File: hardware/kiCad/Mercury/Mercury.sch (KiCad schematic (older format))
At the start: 55 parts

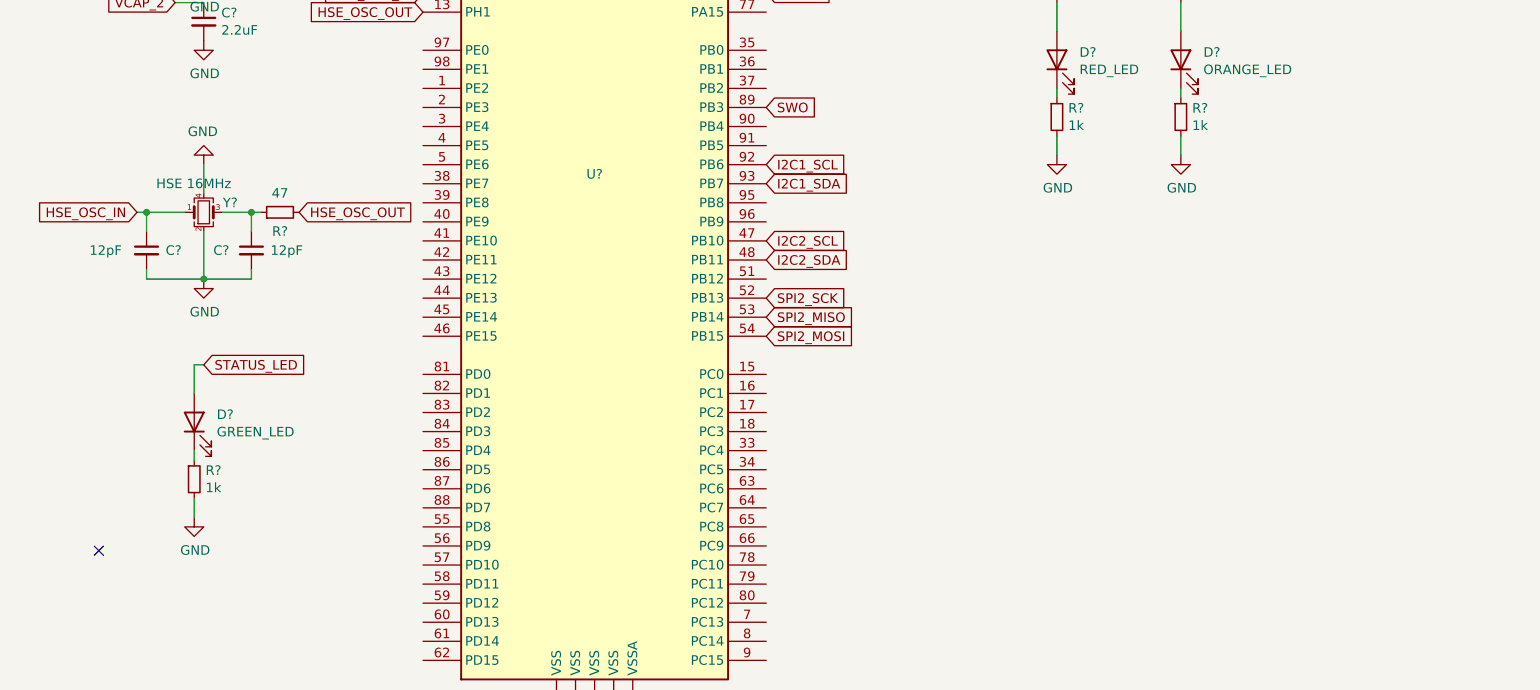
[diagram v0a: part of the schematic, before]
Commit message: Peripherals Added
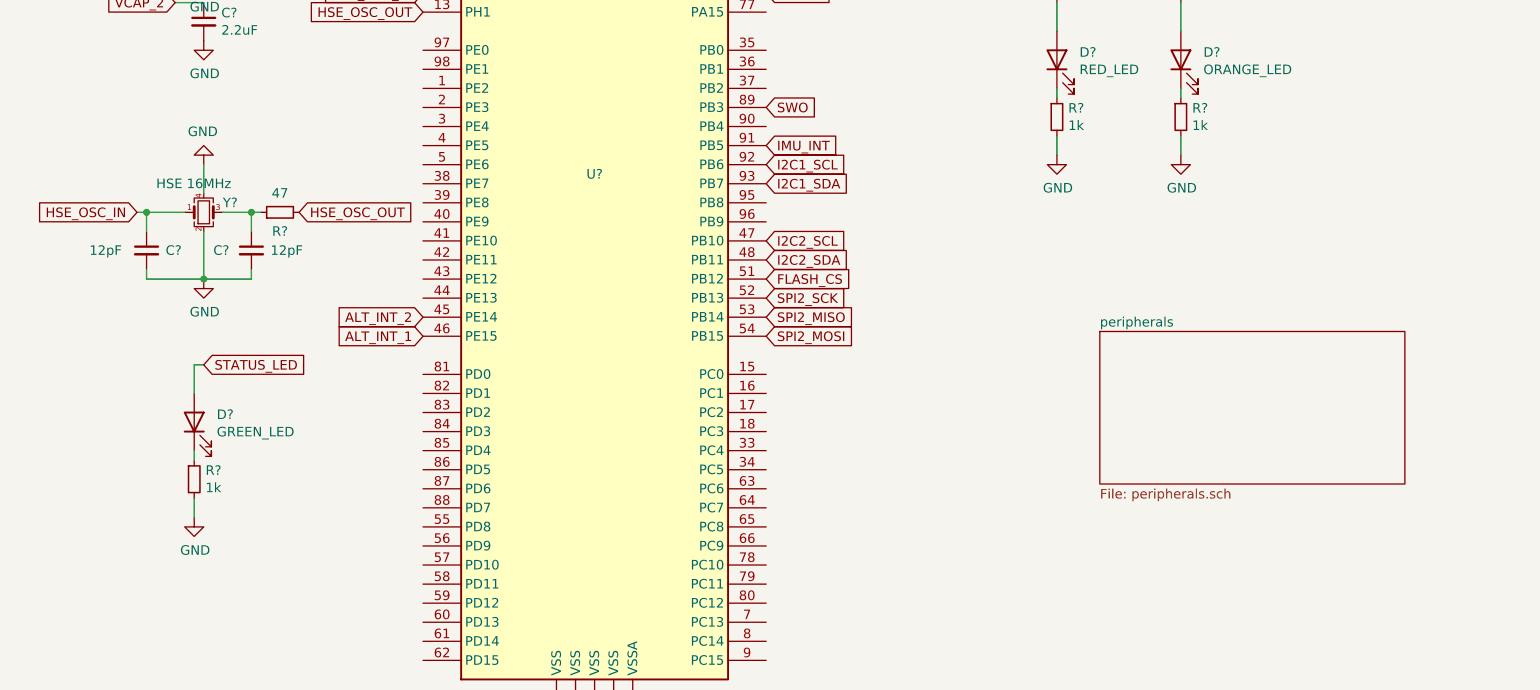
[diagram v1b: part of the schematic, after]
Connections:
- net ALT_INT_2: now reaches U?.45 (PE14)
- net ALT_INT_1: now reaches U?.46 (PE15)
- net FLASH_CS: now reaches U?.51 (PB12)
- net IMU_INT: now reaches U?.91 (PB5)
- no-connect marks 6 -> 5
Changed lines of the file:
@@
 $Descr USLetter 11000 8500
 encoding utf-8
-Sheet 1 1
+Sheet 1 2
 Title "Mercury Avionics Package"
 Date "2020-12-21"
@@
 	0    -1   -1   0
 $EndComp
-NoConn ~ 800  6125
 $Comp
 L Device:LED D?
@@
 	-1   0    0    1
 $EndComp
+$Sheet
+S 6050 4975 1600 800
+U 5FE81F4B
+F0 "peripherals" 50
+F1 "peripherals.sch" 50
+$EndSheet
+Text GLabel 4300 4000 2    50   Input ~ 0
+IMU_INT
+Text GLabel 4300 4700 2    50   Input ~ 0
+FLASH_CS
+Text GLabel 2500 4900 0    50   Input ~ 0
+ALT_INT_2
+Text GLabel 2500 5000 0    50   Input ~ 0
+ALT_INT_1
 $EndSCHEMATC
